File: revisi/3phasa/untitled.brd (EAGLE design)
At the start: 100 x 100 mm, 59 parts, among them J1 U.FL-R-SMT(01), J2 10118193-0001LF, K2 SRD-05VDC-SL-C, Q1 S9013, Q16 MMBT3904, Q17 MMBT3904, Q18 12MHz, U1 AMS1117, U19 CH340G, U2 PC817X2NIP0F, U3 ESP32-WROOM-32D

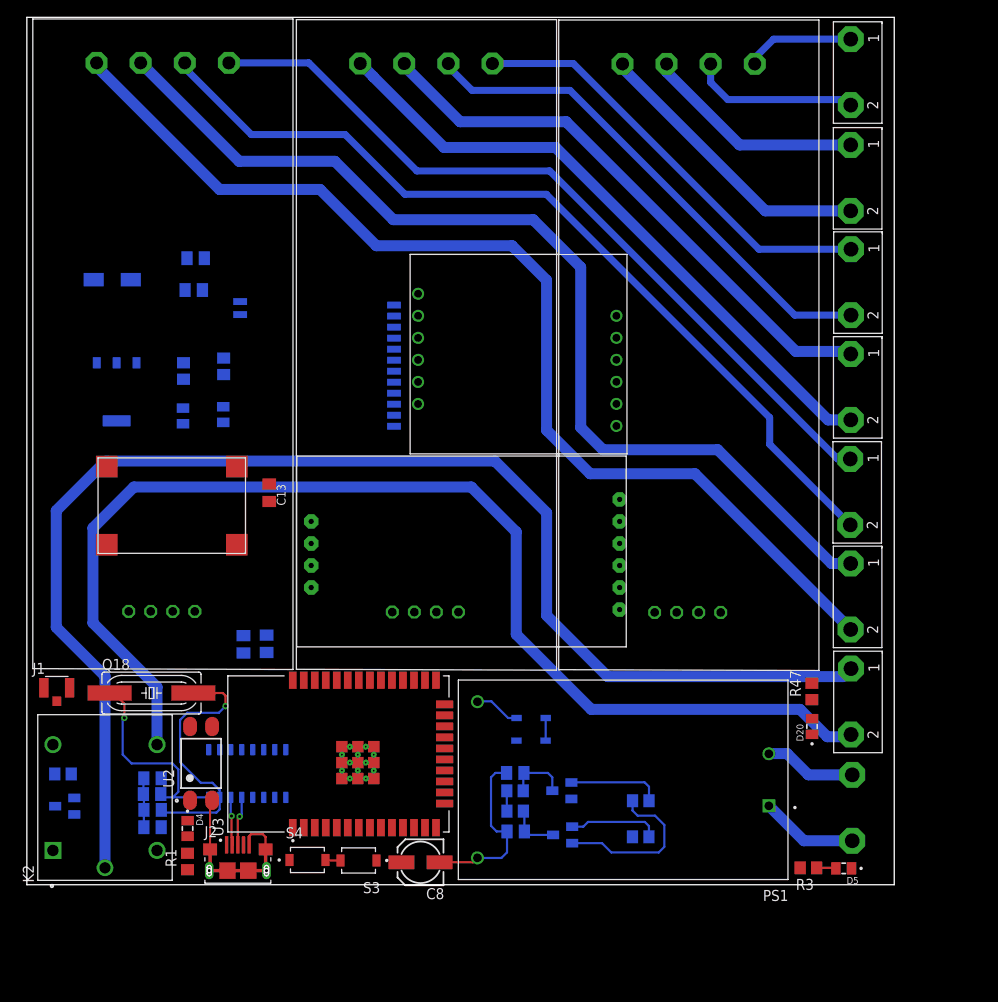
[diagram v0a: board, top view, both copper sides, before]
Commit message: revisi besar-besaran
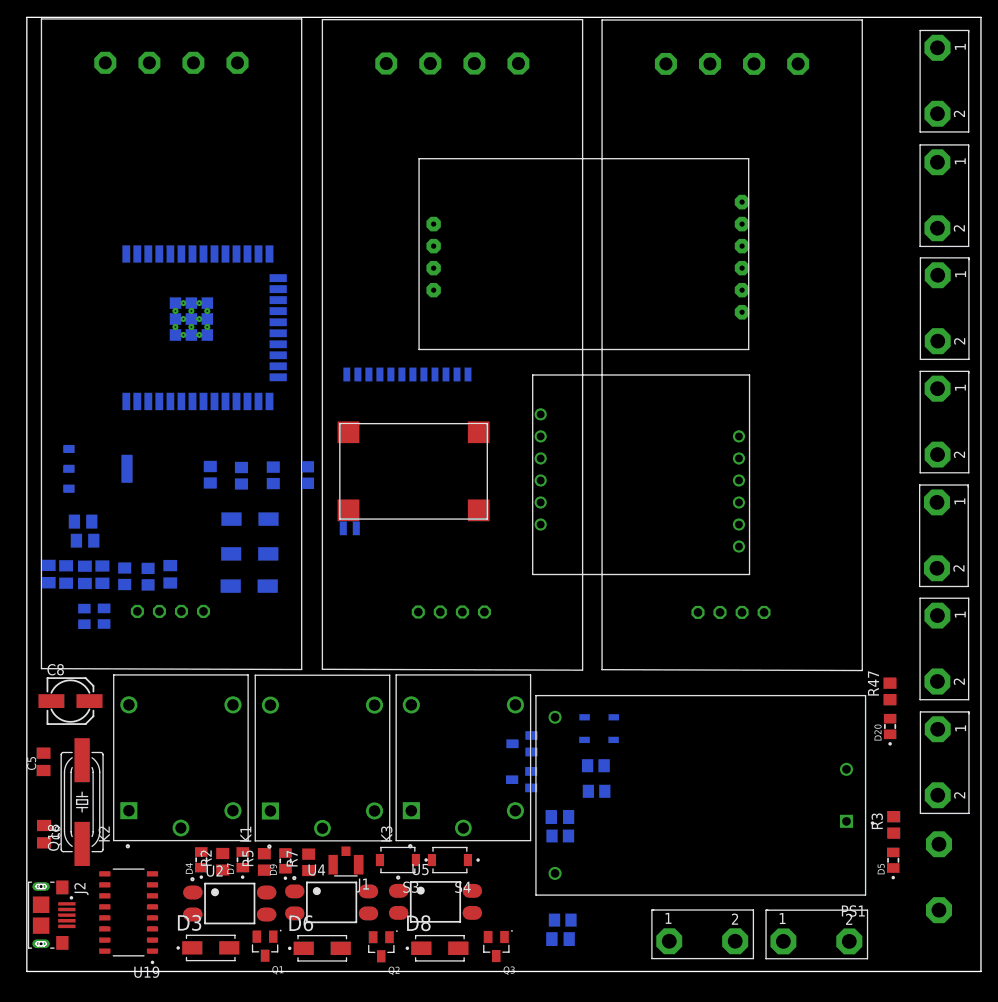
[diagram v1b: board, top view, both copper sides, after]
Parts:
- added D10, D11, D12, D6, D8: US1M-13, US1M-13:DIOM5226X240N
- added D7, D9: SML-LXT0805IW-TR, SML-LXT0805IW-TR:LEDC2012X120N
- added K1, K3: SRD-05VDC-SL-C, SRD-05VDC-SL-C:RELAY_SRD-05VDC-SL-C
- added Q2, Q3: S9013, S9013:SOT95P240X120-3N
- added R4, R6: 330, rcl:R0805
- added R5, R7, R8: 10k, rcl:R0805
- added TB7.10, TB7.9: (no value), TB7.62:TB7.62
- added U4, U5: PC817X2NIP0F, PC817X2NIP0F:SOT254P975X400-4N
- moved D3 77.9 mm to (21.2, -7.29), flipped to the top
- moved U3 52.8 mm to (16.7, 64.2), flipped to the bottom, turned to 270 degrees
- moved R1 44.7 mm to (21.1, 47.3), flipped to the bottom, turned to 270 degrees
- moved C8 44.4 mm to (5.03, 21.2), turned to 0 degrees
- moved J1 39.1 mm to (36.8, 2.32), turned to 180 degrees
- moved C1 38.7 mm to (6.70, 35.7), turned to 90 degrees
- moved RTC1 37.1 mm to (67.2, 78.7)
- moved C2 34.5 mm to (8.71, 35.8), turned to 90 degrees
- moved C9 30.8 mm to (4.52, 35.8), turned to 270 degrees
- moved C10 30.7 mm to (6.49, 41.9)
- moved D18 28.2 mm to (6.64, 30.9)
- moved Q1 28.2 mm to (27.5, -7.08), flipped to the top, turned to 180 degrees
- moved MINI1 28.2 mm to (36.1, 42.2)
- moved R45 26.8 mm to (11.3, 35.6)
- moved C7 26.4 mm to (2.51, 35.8)
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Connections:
- new net N$26: R5.1, U4.4
- new net N$27: Q2.1, U4.3
- new net N$28: D6.A, K1.A2, Q2.3
- new net N$29: K1.COM, TB7.9.T1
- new net N$30: D7.C, U4.1
- new net N$31: D7.A, R4.2
- new net N$32: K1.NO, TB7.9.T2
- new net N$33: R7.1, U5.4
- new net N$34: Q3.1, U5.3
- new net N$35: D8.A, K3.A2, Q3.3
- new net N$36: K3.COM, TB7.10.T1
- new net N$37: D9.C, U5.1
- new net N$38: D9.A, R6.2
- new net N$39: K3.NO, TB7.10.T2
- new net N$40: D10.C, PZEM004T1.TX
- new net N$41: D11.C, PZEM004T2.TX
- new net N$42: D12.C, PZEM004T3.TX
- new net RELAY1: R4.1, U3.9
- new net RELAY2: R6.1, U3.12
- net GND: now also Q2.2, Q3.2, U4.2, U5.2
- net RX_PZEM: now also U3.28; no longer U3.27
- net TX_PZEM: now also D10.A, D11.A, D12.A, R8.1, U3.27; no longer PZEM004T1.TX, PZEM004T2.TX, PZEM004T3.TX, U3.28
- net VCC: now also D6.C, D8.C, K1.A1, K3.A1, R5.2, R7.2, R8.2
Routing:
- net N$9: track 155.1 -> 0.00 mm
- net N$10: track 136.3 -> 0.00 mm
- net N$15: track 124.4 -> 0.00 mm
- net N$16: track 116.6 -> 0.00 mm
- net N$17: track 101.0 -> 0.00 mm
- net N$18: track 90.6 -> 0.00 mm
- net N$14: track 73.6 -> 0.00 mm
- net GND: track 72.3 -> 0.00 mm
- net N$19: track 65.5 -> 0.00 mm
- net N$20: track 58.7 -> 0.00 mm
- net N$21: track 50.2 -> 0.00 mm
- net N$22: track 33.6 -> 0.00 mm
- net N$102: track 30.9 -> 0.00 mm, vias 1 -> 0
- net N$23: track 25.6 -> 0.00 mm
- net N$103: track 24.4 -> 0.00 mm, vias 1 -> 0
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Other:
- board size 100 x 100 mm -> 110 x 110 mm
